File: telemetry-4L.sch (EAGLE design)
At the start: 70 parts, among them SW1 SPST_TACT-KMR2, SW2 PCM12SMTR, U1 ATSAMD21G18A-MUT, U2 SPX3819M5-L-3-0, U3 MCP73831T-2ACI/OT, U4 IRLML6344TRPBF, U5 SIM868, U6 BMP280, U7 MPU-9250, U8 TPS61253YFFR, X1 S2B-PH-SM4-TB(LF)(SN), X2 FC-135 32.7680KA-A3, X3 MF-CON-MICROUSB-RIGHT, X4 104239-1430, X5 U.FL-R-SMT(10), X6 U.FL-R-SMT(10)

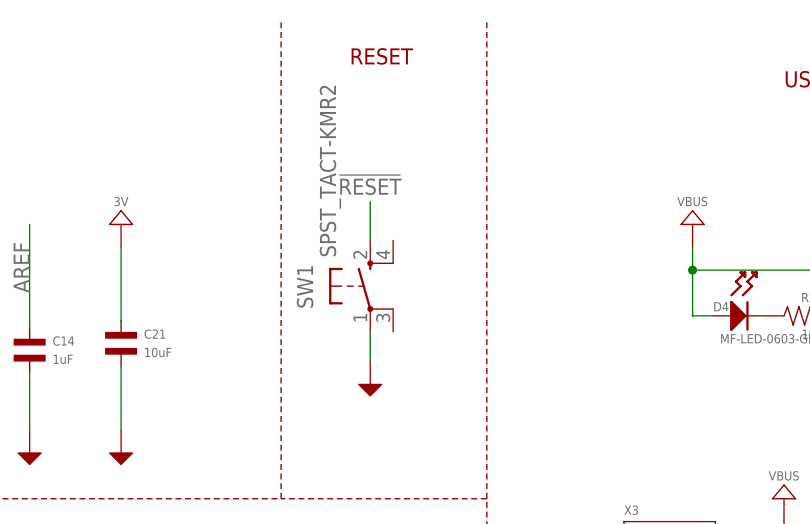
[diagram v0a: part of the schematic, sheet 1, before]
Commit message: small fixes (some very important)
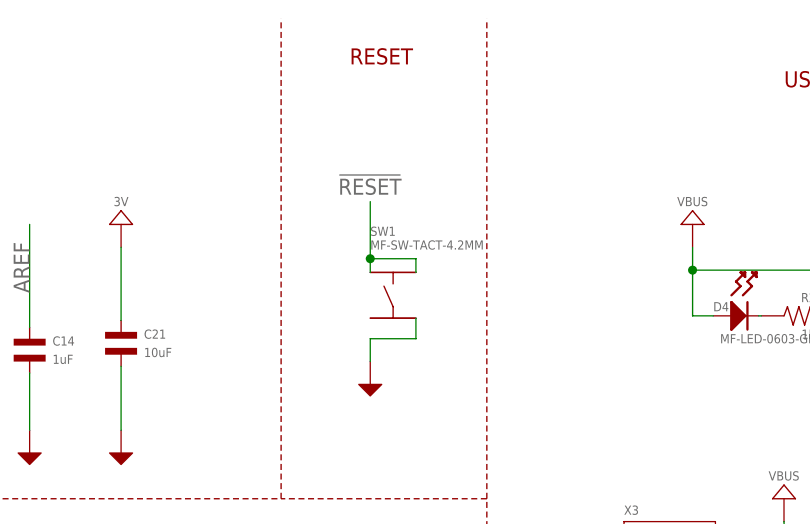
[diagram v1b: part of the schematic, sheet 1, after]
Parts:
- SW1: value SPST_TACT-KMR2 -> MF-SW-TACT-4.2MM; device adafruit:SPST_TACT-KMR2 -> MF_Switches:TACT_4.2MM
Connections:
- net !RESET: now also SW1.P$1, SW1.P$2; no longer SW1.S
- net GND: now also SW1.P$4; no longer SW1.P
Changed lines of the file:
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@@
 <part name="VDD_EXT_2V8" library="MF_Aesthetics" deviceset="POWER_RAIL" device="" value="VDD_EXT_2V8"/>
 <part name="VDD_EXT_2V1" library="MF_Aesthetics" deviceset="POWER_RAIL" device="" value="VDD_EXT_2V8"/>
-<part name="SW1" library="adafruit" deviceset="SPST_TACT" device="-KMR2"/>
+<part name="SW1" library="MF_Switches" deviceset="TACT" device="_4.2MM" value="MF-SW-TACT-4.2MM"/>
 </parts>
 <sheets>
@@
 <instance part="JP3" gate="G$1" x="180.34" y="66.04"/>
 <instance part="5.0V" gate="G$1" x="147.32" y="50.8" rot="R90"/>
-<instance part="SW1" gate="G$1" x="121.666" y="145.542"/>
+<instance part="SW1" gate="G$1" x="124.206" y="144.526"/>
 </instances>
 <busses>
@@
 </segment>
 <segment>
-<wire x1="121.666" y1="140.462" x2="121.666" y2="137.16" width="0.1524" layer="91"/>
 <pinref part="U$47" gate="G$1" pin="P$1"/>
-<pinref part="SW1" gate="G$1" pin="P"/>
+<pinref part="SW1" gate="G$1" pin="P$4"/>
+<wire x1="121.666" y1="139.7" x2="121.666" y2="137.16" width="0.1524" layer="91"/>
+<wire x1="126.746" y1="141.986" x2="126.746" y2="139.7" width="0.1524" layer="91"/>
+<wire x1="126.746" y1="139.7" x2="121.666" y2="139.7" width="0.1524" layer="91"/>
 </segment>
 <segment>
@@
 <segment>
 <label x="118.11" y="155.702" size="1.778" layer="95"/>
-<wire x1="121.666" y1="154.94" x2="121.666" y2="150.622" width="0.1524" layer="91"/>
-<pinref part="SW1" gate="G$1" pin="S"/>
-</segment>
-<segment>
+<wire x1="121.666" y1="154.94" x2="121.666" y2="148.59" width="0.1524" layer="91"/>
+<pinref part="SW1" gate="G$1" pin="P$2"/>
+<wire x1="126.746" y1="147.066" x2="126.746" y2="148.59" width="0.1524" layer="91"/>
+<wire x1="126.746" y1="148.59" x2="121.666" y2="148.59" width="0.1524" layer="91"/>
+<pinref part="SW1" gate="G$1" pin="P$1"/>
+<wire x1="121.666" y1="147.066" x2="121.666" y2="148.59" width="0.1524" layer="91"/>
+<junction x="121.666" y="148.59"/>
+</segment>
+<segment>
